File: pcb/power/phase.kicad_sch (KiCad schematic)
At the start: 20 parts, among them J1 Conn_02x02_Odd_Even, J2 Conn_02x03_Odd_Even, Q1 SP010N01BGHTO, Q2 SP010N01BGHTO, Q3 SP010N01BGHTO, Q4 SP010N01BGHTO, U1 INA181

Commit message: Update shunts
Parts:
- R1, R2, R3: footprint Resistor_SMD:R_2512_6332Metric -> Resistor_SMD:R_4020_10251Metric; LCSC C5123666 -> C2927603
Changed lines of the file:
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@@
 			)
 		)
-		(property "Footprint" "Resistor_SMD:R_2512_6332Metric"
+		(property "Footprint" "Resistor_SMD:R_4020_10251Metric"
 			(at 49.022 102.87 90)
 			(effects
@@
 			)
 		)
-		(property "LCSC" "C5123666"
+		(property "LCSC" "C2927603"
 			(at 50.8 102.87 0)
 			(effects
@@
 			)
 		)
-		(property "Footprint" "Resistor_SMD:R_2512_6332Metric"
+		(property "Footprint" "Resistor_SMD:R_4020_10251Metric"
 			(at 41.402 102.87 90)
 			(effects
@@
 			)
 		)
-		(property "LCSC" "C5123666"
+		(property "LCSC" "C2927603"
 			(at 43.18 102.87 0)
 			(effects
@@
 			)
 		)
-		(property "Footprint" "Resistor_SMD:R_2512_6332Metric"
+		(property "Footprint" "Resistor_SMD:R_4020_10251Metric"
 			(at 33.782 102.87 90)
 			(effects
@@
 			)
 		)
-		(property "LCSC" "C5123666"
+		(property "LCSC" "C2927603"
 			(at 35.56 102.87 0)
 			(effects

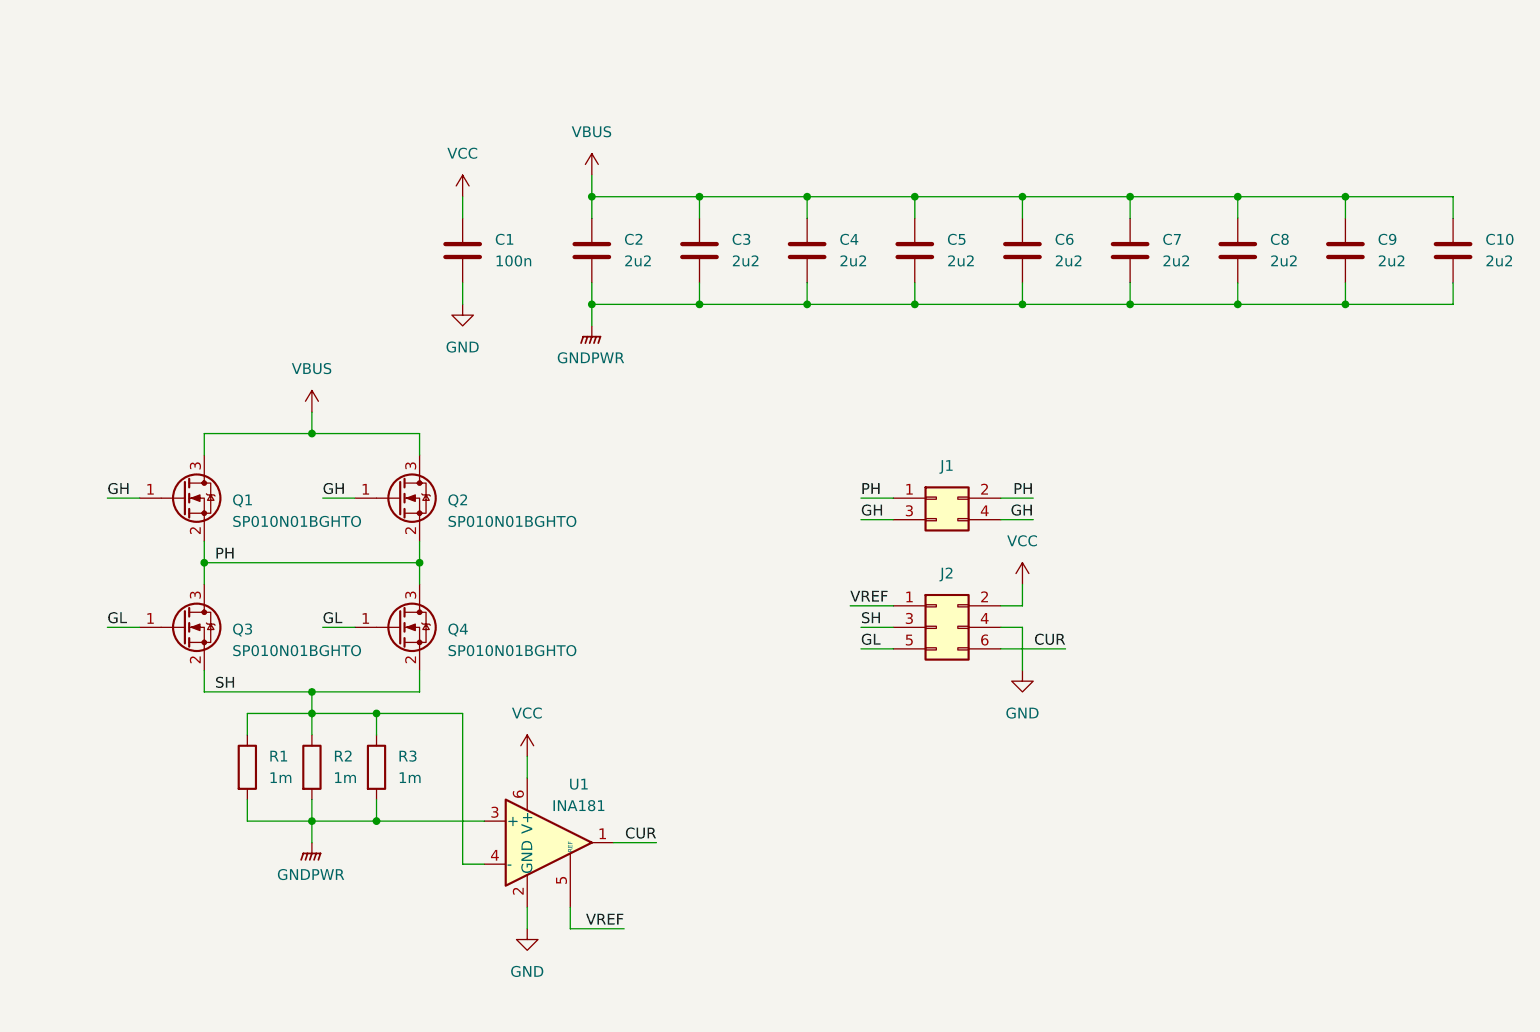
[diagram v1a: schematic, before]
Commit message: Finish rev 1
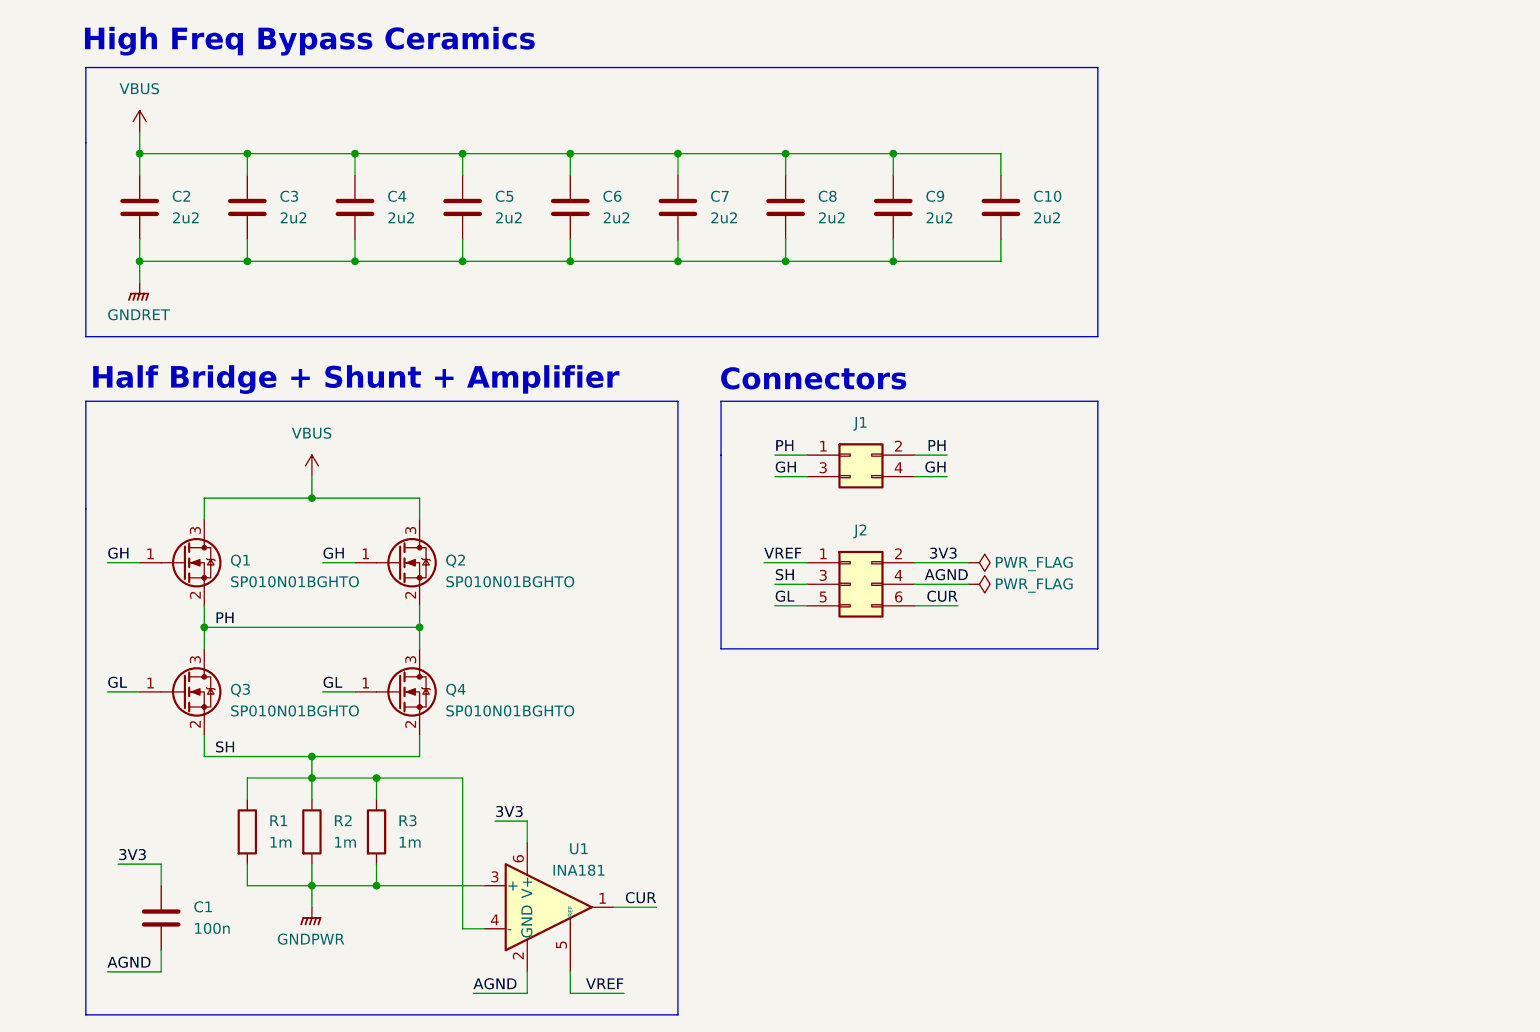
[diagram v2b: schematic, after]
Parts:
- removed Q1, Q2, Q3, Q4: SP010N01BGHTO, Package_TO_SOT_SMD:Infineon_PG-HSOF-8-1, symbol Transistor_FET:IPT015N10N5
- added Q1, Q2, Q3, Q4: SP010N01BGHTO, Package_TO_SOT_SMD:Infineon_PG-HSOF-8-1, symbol User_Symbols:SP010N01BGHTO
- C1: LCSC C1525 -> C307331
- R1, R2, R3: footprint Resistor_SMD:R_4020_10251Metric -> User_Footprints:R_Shunt_3921
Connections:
- net GH: now also Q1.1 (G), Q2.1 (G)
- net GL: now also Q3.1 (G), Q4.1 (G)
- net GNDPWR: no longer C10.2, C2.2, C3.2, C4.2, C5.2, C6.2, C7.2, C8.2, C9.2
- net PH: now also Q1.2 (S), Q2.2 (S), Q3.3 (D), Q4.3 (D)
- net SH: now also Q3.2 (S), Q4.2 (S)
- net VBUS: now also Q1.3 (D), Q2.3 (D)
- net GND renamed AGND
- net VCC renamed 3V3
- new net GNDRET: C10.2, C2.2, C3.2, C4.2, C5.2, C6.2, C7.2, C8.2, C9.2
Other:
- note added: "Connectors"
- note added: "Half Bridge + Shunt + Amplifier"
- note added: "High Freq Bypass Ceramics"
- moved on the sheet: C1, C10, C2, C3, C4, C5, C6, C7, C8, C9, J1, J2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
